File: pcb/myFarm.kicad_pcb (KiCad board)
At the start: 2 copper layers, 63.5 x 52.1 mm, 19 parts, among them J0 POWER, J1 LED, J10 GENERAL, J11 RXTX, J12 VALVE OUT, J13 VALVE OUT, J14 VALVE OUT, J15 SELECTOR, J2 SENSOR, J3 SW_LED, J4 RELAY, J5 POWER DRIVE, J6 JUMPER, J7 SUPPLY, J8 Reset, J9 VAVLE IN, U1 WeMos_D1_mini, U2 MCP23017_MODULE, U3 DS1832S+

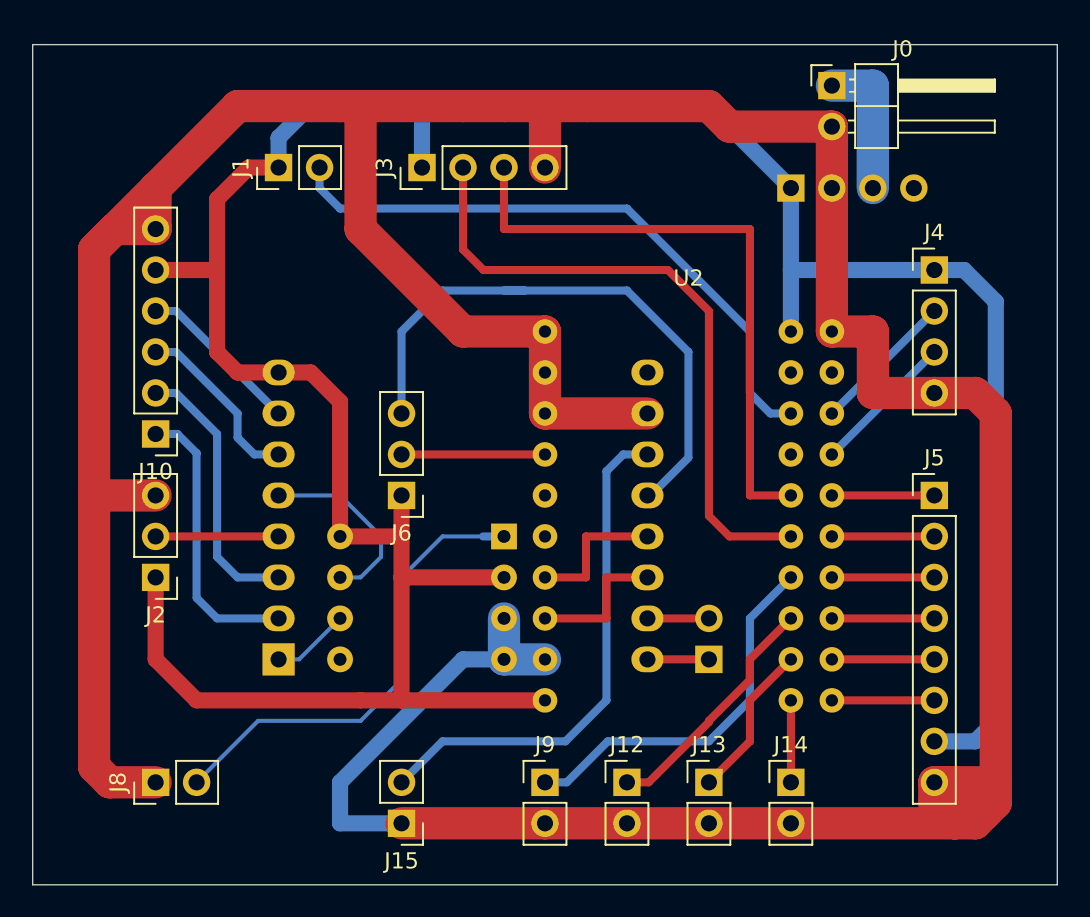
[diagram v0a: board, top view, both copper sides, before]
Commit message: update pcb
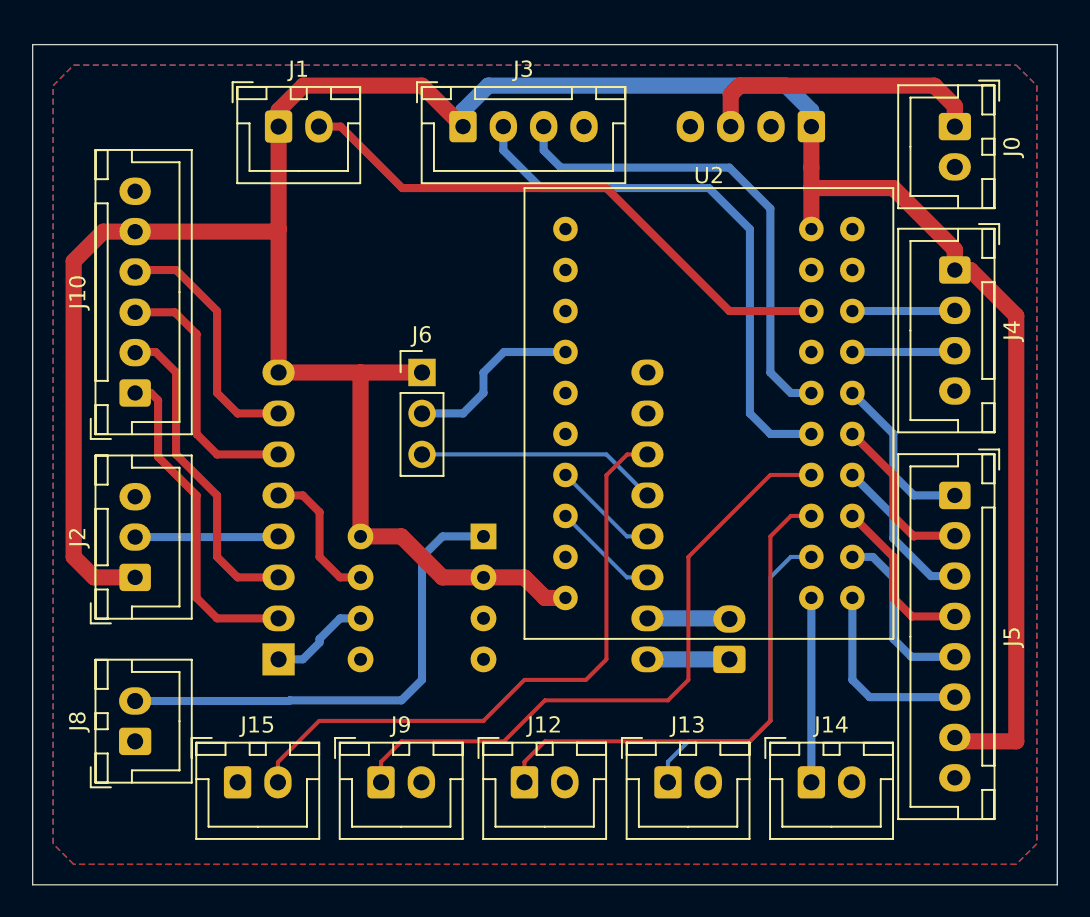
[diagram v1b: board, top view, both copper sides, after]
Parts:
- J0: footprint Connector_PinHeader_2.54mm:PinHeader_1x02_P2.54mm_Horizontal -> Connector_JST:JST_XH_B2B-XH-A_1x02_P2.50mm_Vertical
- J1, J11, J12, J13, J14, J15, J8, J9: footprint Connector_PinHeader_2.54mm:PinHeader_1x02_P2.54mm_Vertical -> Connector_JST:JST_XH_B2B-XH-A_1x02_P2.50mm_Vertical
- J10: footprint Connector_PinHeader_2.54mm:PinHeader_1x06_P2.54mm_Vertical -> Connector_JST:JST_XH_B6B-XH-A_1x06_P2.50mm_Vertical
- J2: footprint Connector_PinHeader_2.54mm:PinHeader_1x03_P2.54mm_Vertical -> Connector_JST:JST_XH_B3B-XH-A_1x03_P2.50mm_Vertical
- J3, J4: footprint Connector_PinHeader_2.54mm:PinHeader_1x04_P2.54mm_Vertical -> Connector_JST:JST_XH_B4B-XH-A_1x04_P2.50mm_Vertical
- J5: footprint Connector_PinHeader_2.54mm:PinHeader_1x08_P2.54mm_Vertical -> Connector_JST:JST_XH_B8B-XH-A_1x08_P2.50mm_Vertical
- J7: footprint Module:POWER_SUPPLY_MODULE -> Connector_JST:JST_XH_B4B-XH-A_1x04_P2.50mm_Vertical
- U3: footprint Package_DIP:DIP-8_W10.16mm -> Package_DIP:DIP-8_W7.62mm_Socket
- moved J15 10.5 mm to (74.9, 94.0), turned to 0 degrees
- moved J9 10.2 mm to (83.8, 94.0)
- moved J0 8.03 mm to (119.4, 53.3), turned to 270 degrees
- moved J6 7.73 mm to (86.4, 68.6), turned to 0 degrees
- moved U2 6.48 mm to (104.1, 55.9)
- moved J12 6.35 mm to (92.7, 94.0)
- moved J7 4.02 mm to (110.5, 53.3), turned to 180 degrees
- moved J3 3.59 mm to (88.9, 53.3), turned to 0 degrees
- moved J10 2.84 mm to (68.6, 69.8), turned to 90 degrees
- moved J8 2.84 mm to (68.6, 91.4)
- moved J13 2.54 mm to (101.6, 94.0)
- moved J1 2.54 mm to (77.5, 53.3), turned to 0 degrees
- moved J11 1.27 mm to (105.4, 86.4), turned to 90 degrees
- moved J14 1.27 mm to (110.5, 94.0)
- moved J2 1.27 mm to (68.6, 81.3), turned to 90 degrees
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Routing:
- net GNDREF: track 260.2 -> 0.00 mm
- net Net-(J6-Pad3): track 37.0 -> 15.0 mm
- net Net-(J9-Pad1): track 23.5 -> 40.8 mm
- net Net-(J12-Pad1): track 15.2 -> 32.1 mm
- net Net-(J13-Pad1): track 9.72 -> 20.6 mm
- net Net-(J0-Pad1): track 8.89 -> 17.9 mm
- net Net-(J3-Pad3): track 38.1 -> 30.2 mm
- net Net-(J15-Pad2): track 32.0 -> 38.7 mm
- net Net-(J14-Pad1): track 5.08 -> 11.4 mm
- net Net-(J3-Pad2): track 40.2 -> 34.5 mm
- net Net-(J5-Pad6): track 6.35 -> 11.9 mm
- net Net-(J10-Pad4): track 10.3 -> 15.6 mm
- net Net-(J10-Pad3): track 11.1 -> 16.2 mm
- net Net-(J5-Pad5): track 6.35 -> 11.1 mm
- net Net-(J1-Pad1): track 181.3 -> 177.1 mm
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- added copper zone on B.Cu, net GNDREF
- added copper zone on F.Cu, net GNDREF
